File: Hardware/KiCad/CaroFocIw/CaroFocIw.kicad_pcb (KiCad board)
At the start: 4 copper layers, 140 x 70 mm, 97 parts, among them J1 Conn_01x02, J10 Conn_01x05, J11 Conn_01x05, J12 Conn_01x02, J13 Conn_01x02, J14 Conn_01x03, J15 Conn_01x03, J16 Conn_01x03, J17 Conn_01x05, J18 Conn_01x05, J19 Conn_01x02, J2 Conn_01x01, J3 Conn_01x01, J4 Conn_01x01, J5 Conn_01x01, J6 Conn_01x02, J7 Conn_01x03, J8 Conn_01x03, J9 Conn_01x03, Q1 Q_NMOS_SGD, Q2 Q_NMOS_SGD, Q3 Q_NMOS_SGD, Q4 Q_NMOS_SGD, Q5 Q_NMOS_SGD, Q6 Q_NMOS_SGD, U1 TCAN332, U2 STM32F405RGTx, U3 TLE7185-1E, U4 ACS711xEXLT-15AB, U5 AS5048A, U6 ACS711xEXLT-15AB, U7 ACS711xEXLT-15AB, U8 LMR16006YQ3

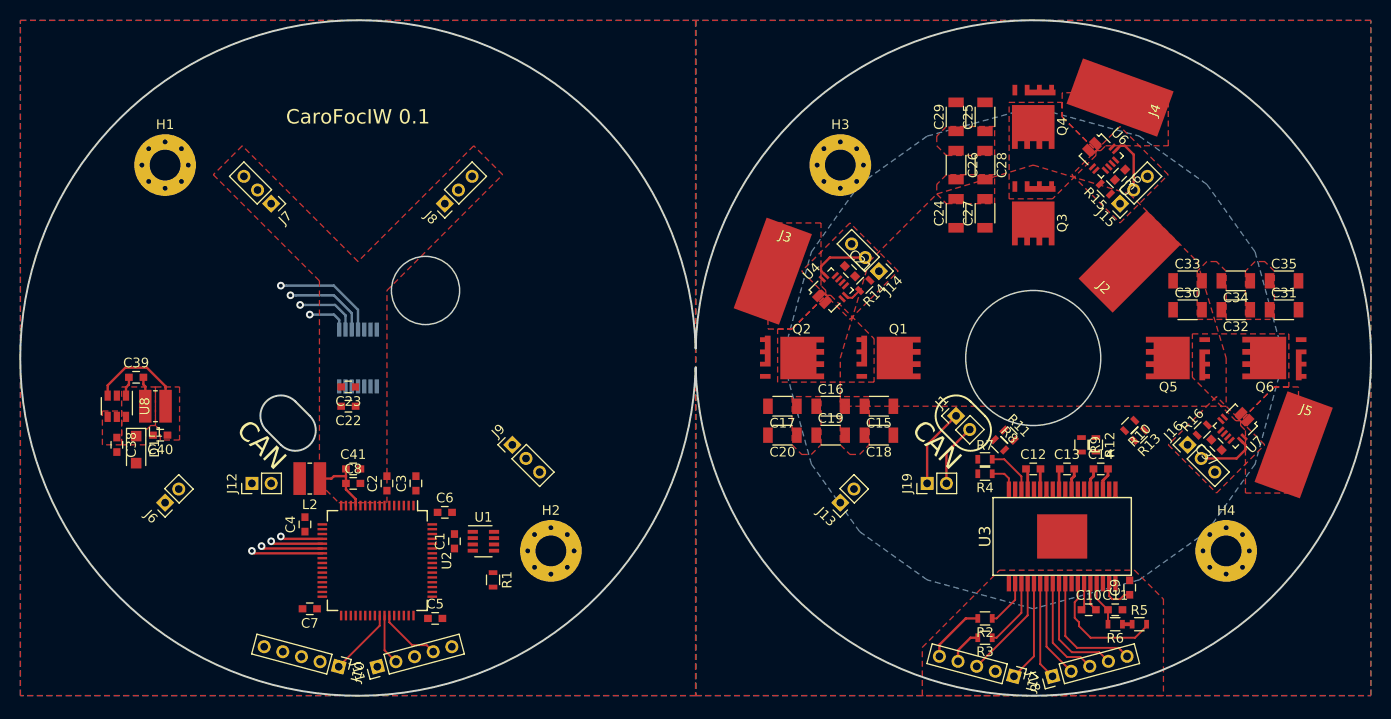
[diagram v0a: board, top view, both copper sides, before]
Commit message: Some more layout work
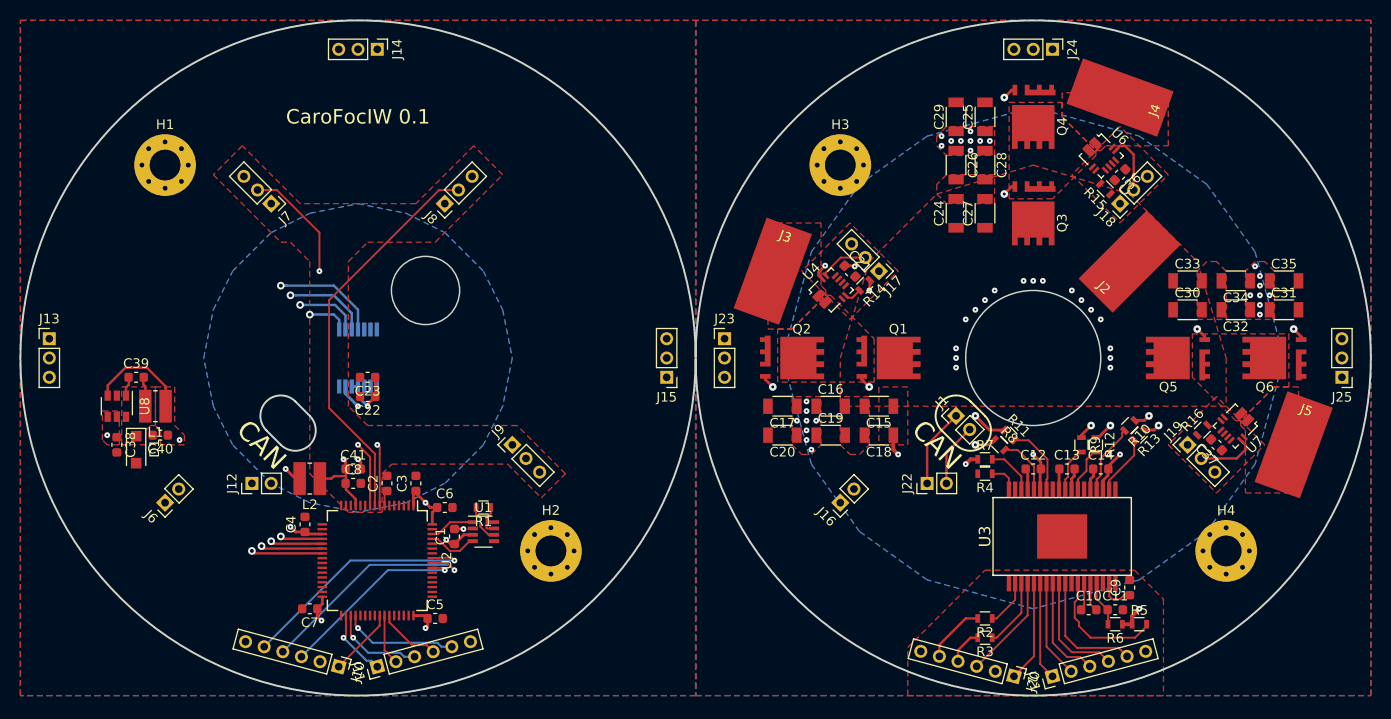
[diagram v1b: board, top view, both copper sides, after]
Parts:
- added J20: Conn_01x06, Connector_PinHeader_2.00mm:PinHeader_1x06_P2.00mm_Vertical, F.Cu at (208.0, 158.0)
- added J21: Conn_01x06, Connector_PinHeader_2.00mm:PinHeader_1x06_P2.00mm_Vertical, F.Cu at (212.0, 158.0)
- added J22: Conn_01x02, Connector_PinHeader_2.00mm:PinHeader_1x02_P2.00mm_Vertical, F.Cu at (199.0, 138.0)
- added J23: Conn_01x03, Connector_PinHeader_2.00mm:PinHeader_1x03_P2.00mm_Vertical, F.Cu at (178.0, 123.0)
- added J24: Conn_01x03, Connector_PinHeader_2.00mm:PinHeader_1x03_P2.00mm_Vertical, F.Cu at (212.0, 93.0)
- added J25: Conn_01x03, Connector_PinHeader_2.00mm:PinHeader_1x03_P2.00mm_Vertical, F.Cu at (242.0, 127.0)
- C1, C10, C11, C12, C13, C14, C2, C21, C22, C23, C3, C36, C37, C38, C39, C4, C40, C41, C5, C6, C7, C8, C9: footprint Capacitors_SMD:C_0603 -> Capacitor_SMD:C_0603_1608Metric
- J10, J11: value Conn_01x05 -> Conn_01x06; footprint Pin_Headers:Pin_Header_Straight_1x05_Pitch2.00mm -> Connector_PinHeader_2.00mm:PinHeader_1x06_P2.00mm_Vertical
- J12, J6: footprint Pin_Headers:Pin_Header_Straight_1x02_Pitch2.00mm -> Connector_PinHeader_2.00mm:PinHeader_1x02_P2.00mm_Vertical
- J13, J19: value Conn_01x02 -> Conn_01x03; footprint Pin_Headers:Pin_Header_Straight_1x02_Pitch2.00mm -> Connector_PinHeader_2.00mm:PinHeader_1x03_P2.00mm_Vertical
- J14, J15, J7, J8, J9: footprint Pin_Headers:Pin_Header_Straight_1x03_Pitch2.00mm -> Connector_PinHeader_2.00mm:PinHeader_1x03_P2.00mm_Vertical
- J16: value Conn_01x03 -> Conn_01x02; footprint Pin_Headers:Pin_Header_Straight_1x03_Pitch2.00mm -> Connector_PinHeader_2.00mm:PinHeader_1x02_P2.00mm_Vertical
- J17, J18: value Conn_01x05 -> Conn_01x03; footprint Pin_Headers:Pin_Header_Straight_1x05_Pitch2.00mm -> Connector_PinHeader_2.00mm:PinHeader_1x03_P2.00mm_Vertical
- moved J13 83.7 mm to (108.0, 123.0), turned to 0 degrees
- moved J14 56.9 mm to (142.0, 93.0), turned to 270 degrees
- moved J15 50.3 mm to (172.0, 127.0), turned to 180 degrees
- moved J18 49.5 mm to (219.0, 109.0), turned to 135 degrees
- moved J17 44.3 mm to (194.0, 116.0), turned to 225 degrees
- moved J16 36.5 mm to (190.0, 140.0), turned to 135 degrees
- moved J19 27.3 mm to (226.0, 134.0), turned to 45 degrees
- moved R1 7.57 mm to (153.0, 140.5), turned to 180 degrees
- moved C22 2.24 mm to (141.0, 129.0)
- moved C23 2.24 mm to (141.0, 127.0)
- moved U1 1.00 mm to (153.0, 143.0)
- moved C1 0.50 mm to (150.0, 143.5)
- moved C6 0.50 mm to (149.0, 140.5)
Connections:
- J13 pad 1: GNDPWR -> GNDPWR_A
- J13 pad 2: +BATT -> GNDPWR_A
- J14 pad 1: AGND_U -> GNDPWR_A
- J14 pad 2: /CurrentSensingU/AnalogOut -> GNDPWR_A
- J14 pad 3: 3.3VA_U -> GNDPWR_A
- J15 pad 1: AGND_V -> GNDPWR_A
- J15 pad 2: /CurrentSensingV/AnalogOut -> GNDPWR_A
- J15 pad 3: 3.3VA_V -> GNDPWR_A
- J16 pad 1: AGND_W -> GNDPWR
- J16 pad 2: /CurrentsensingW/AnalogOut -> +BATT
- J17 pad 1: /GateDriver/~LogicUH -> AGND_U
- J17 pad 2: GND_B -> /CurrentSensingU/AnalogOut
- J17 pad 3: /GateDriver/LogicGdEna -> 3.3VA_U
- J18 pad 1: /GateDriver/LogicUL -> AGND_V
- J18 pad 2: /GateDriver/~LogicVH -> /CurrentSensingV/AnalogOut
- J18 pad 3: /GateDriver/LogicVL -> 3.3VA_V
- J19 pad 1: /PcbToPcbConnector/CanHB -> AGND_W
- J19 pad 2: /PcbToPcbConnector/CanLB -> /CurrentsensingW/AnalogOut
- U2 pad 55: /MCU/~GateDriverErr1 -> /MCU/GateDriverEnable
- U2 pad 56: /MCU/~GateDriverErr2 -> /MCU/~GateDriverErr1
- U2 pad 57: /MCU/GateDriverEnable -> /MCU/~GateDriverErr2
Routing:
- net /HalfBridgeV/GateL: track 0.00 -> 43.6 mm, vias 0 -> 2
- net /MCU/CurrentV: track 0.00 -> 41.4 mm
- net /MCU/CurrentU: track 0.00 -> 39.1 mm, vias 0 -> 2
- net +BATT: track 1.00 -> 38.2 mm, vias 0 -> 45
- net /HalfBridgeV/GateH: track 0.00 -> 33.0 mm, vias 0 -> 2
- net /HalfBridgeU/GateL: track 0.00 -> 28.1 mm, vias 0 -> 2
- net +3V3: track 10.7 -> 38.1 mm, vias 0 -> 8
- net /MCU/~GateDriverErr2: track 0.00 -> 25.9 mm, vias 0 -> 1
- net /MCU/CurrentW: track 0.00 -> 24.8 mm, vias 0 -> 1
- net /MCU/~GateDriverErr1: track 0.00 -> 24.4 mm, vias 0 -> 1
- net /HalfBridgeW/GateL: track 0.00 -> 21.2 mm, vias 0 -> 2
- net /MCU/GateDriverEnable: track 0.00 -> 20.0 mm, vias 0 -> 1
- net /HalfBridgeU/GateH: track 0.00 -> 17.1 mm, vias 0 -> 2
- net /HalfBridgeW/GateH: track 0.00 -> 14.2 mm, vias 0 -> 2
- net /MCU/LogicWL: track 0.00 -> 11.9 mm, vias 0 -> 1
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- added copper zone on In2.Cu, net +3V3
- added copper zone on In2.Cu, net +BATT
- added copper zone on In1.Cu, net /CurrentSensingU/PhaseIn
- added copper zone on In1.Cu, net /CurrentSensingV/PhaseOut
- added copper zone on In1.Cu, net /CurrentsensingW/PhaseIn
- added copper zone on F.Cu, net BattA
- added copper zone on B.Cu, net GND
- added copper zone on In1.Cu, net GNDPWR
- added copper zone on In2.Cu, net GNDPWR
- added copper zone on In1.Cu, net GND_B
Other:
- outline, holes or cut-outs redrawn
